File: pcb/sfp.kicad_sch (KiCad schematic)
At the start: 5 parts, among them J1 SFP, U1 GW1N-6&9_QN48

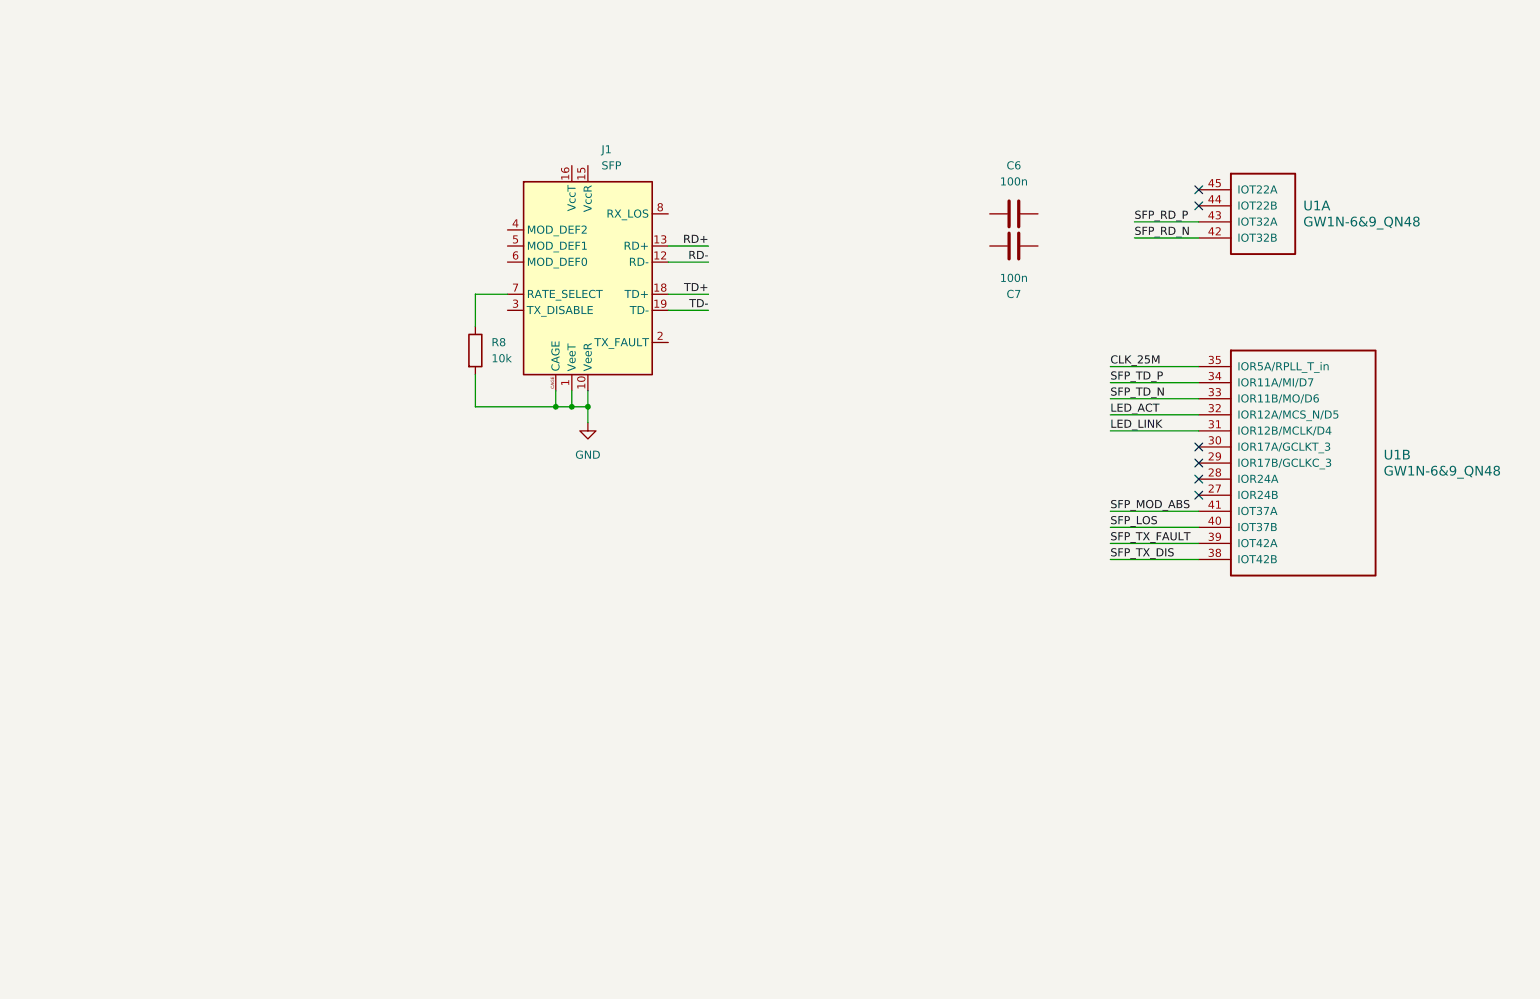
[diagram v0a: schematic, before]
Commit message: pcb: schemat rev. A
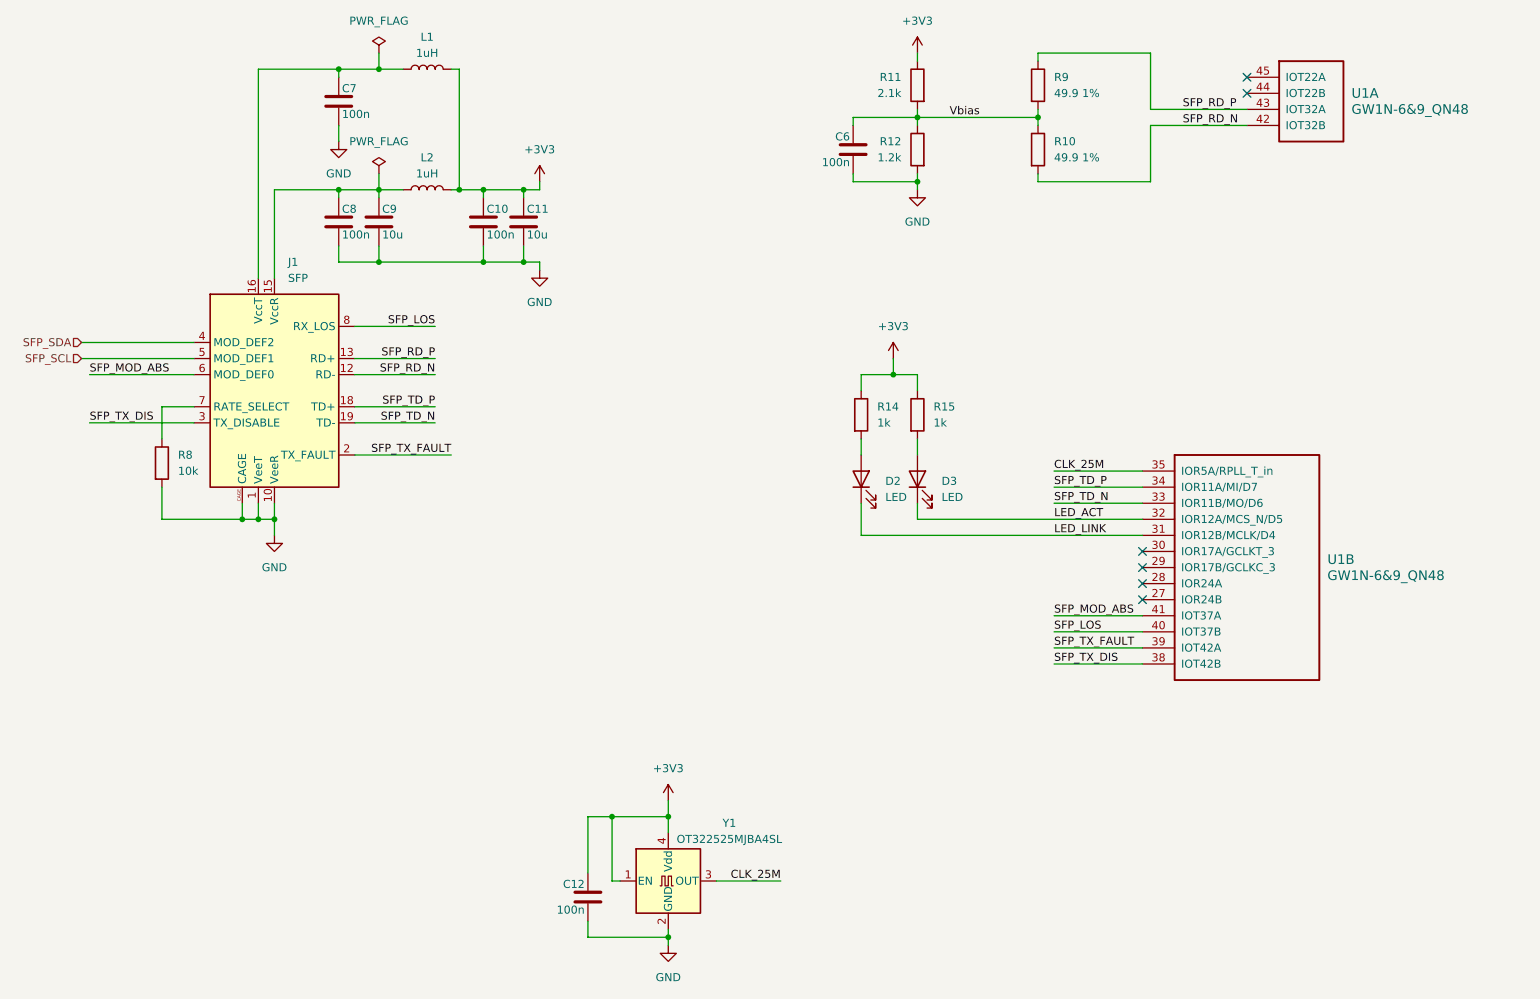
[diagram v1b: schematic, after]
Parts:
- added C10, C12, C8: 100n, Capacitor_SMD:C_0603_1608Metric, symbol Device:C
- added C11, C9: 10u, Capacitor_SMD:C_0603_1608Metric, symbol Device:C
- added D2, D3: LED, LED_SMD:LED_0603_1608Metric, symbol Device:LED
- added L1, L2: 1uH, Inductor_SMD:L_0805_2012Metric, symbol Device:L
- added R10, R9: 49.9 1%, Resistor_SMD:R_0402_1005Metric, symbol Device:R
- added R11: 2.1k, Resistor_SMD:R_0603_1608Metric, symbol Device:R
- added R12: 1.2k, Resistor_SMD:R_0603_1608Metric, symbol Device:R
- added R14, R15: 1k, Resistor_SMD:R_0603_1608Metric, symbol Device:R
- added Y1: OT322525MJBA4SL, Oscillator:Oscillator_SMD_Abracon_ASE-4Pin_3.2x2.5mm, symbol Oscillator:ASE-xxxMHz
- C6, C7: footprint Capacitor_SMD:C_0402_1005Metric -> Capacitor_SMD:C_0603_1608Metric
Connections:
- net RD+ is gone; now on net SFP_RD_P: J1.13 (RD+)
- net RD- is gone; now on net SFP_RD_N: J1.12 (RD-)
- net TD+ is gone; now on net SFP_TD_P: J1.18 (TD+)
- net TD- is gone; now on net SFP_TD_N: J1.19 (TD-)
- net CLK_25M: now also Y1.3 (OUT)
- net GND: now also C6.2, C7.2, C10.2, C11.2, C12.2, C8.2, C9.2, R12.2, Y1.2 (GND)
- net LED_ACT: now also D3.1 (K)
- net LED_LINK: now also D2.1 (K)
- net SFP_LOS: now also J1.8 (RX_LOS)
- net SFP_MOD_ABS: now also J1.6 (MOD_DEF0)
- net SFP_RD_N: now also R10.2
- net SFP_RD_P: now also R9.1
- net SFP_TX_DIS: now also J1.3 (TX_DISABLE)
- net SFP_TX_FAULT: now also J1.2 (TX_FAULT)
- net Vbias: now reaches C6.1
- net Vbias: now also R10.1, R11.2, R12.1, R9.2
- net at C7.1: now also J1.16 (VccT), L1.1
- net at J1.15 (VccR): now also C8.1, C9.1, L2.1
- net SFP_SDA: now reaches J1.4 (MOD_DEF2)
- net SFP_SCL: now reaches J1.5 (MOD_DEF1)
- new net: D3.2 (A), R15.2
- new net: D2.2 (A), R14.2
- new net +3V3: C10.1, C11.1, C12.1, L1.2, L2.2, R11.1, R14.1, R15.1, Y1.1 (EN), Y1.4 (Vdd)
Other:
- moved on the sheet: J1, R8, U1A, U1B
